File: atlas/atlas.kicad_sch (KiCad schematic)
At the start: 0 parts

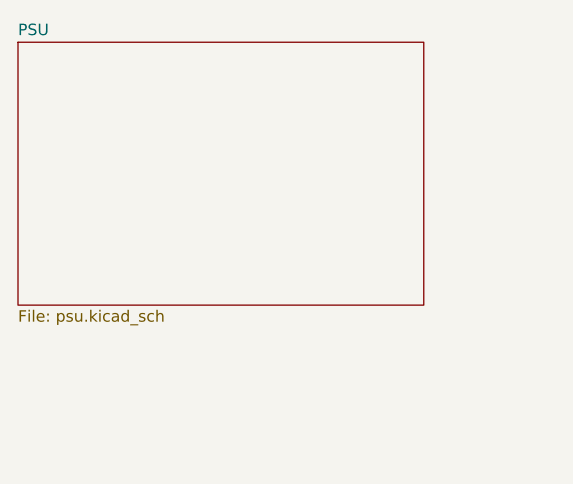
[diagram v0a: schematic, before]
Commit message: sensor supply
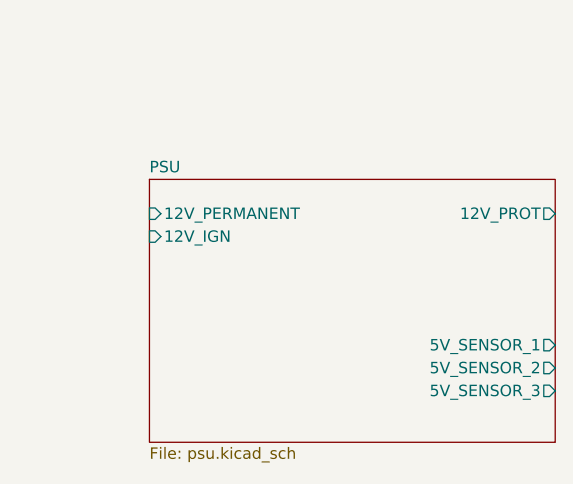
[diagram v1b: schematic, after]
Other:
- sheet PSU ports: added 12V_IGN, 12V_PERMANENT, 12V_PROT, 5V_SENSOR_1, 5V_SENSOR_2, 5V_SENSOR_3; removed none
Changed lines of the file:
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@@
     (rev "a")
   )
-  (sheet (at 20.32 17.78) (size 45.085 29.21) (fields_autoplaced)
+  (sheet (at 34.925 33.02) (size 45.085 29.21) (fields_autoplaced)
     (stroke (width 0.0006) (type solid) (color 0 0 0 0))
     (fill (color 0 0 0 0.0000))
-    (property "Sheet name" "PSU" (id 0) (at 20.32 17.1443 0)
+    (property "Sheet name" "PSU" (id 0) (at 34.925 32.3843 0)
       (effects (font (size 1.27 1.27)) (justify left bottom))
     )
-    (property "Sheet file" "psu.kicad_sch" (id 1) (at 20.32 47.4987 0)
+    (property "Sheet file" "psu.kicad_sch" (id 1) (at 34.925 62.7387 0)
       (effects (font (size 1.27 1.27)) (justify left top))
+    )
+    (pin "12V_PERMANENT" input (at 34.925 36.83 180)
+      (effects (font (size 1.27 1.27)) (justify left))
+    )
+    (pin "12V_IGN" input (at 34.925 39.37 180)
+      (effects (font (size 1.27 1.27)) (justify left))
+    )
+    (pin "12V_PROT" output (at 80.01 36.83 0)
+      (effects (font (size 1.27 1.27)) (justify right))
+    )
+    (pin "5V_SENSOR_1" output (at 80.01 51.435 0)
+      (effects (font (size 1.27 1.27)) (justify right))
+    )
+    (pin "5V_SENSOR_3" output (at 80.01 56.515 0)
+      (effects (font (size 1.27 1.27)) (justify right))
+    )
+    (pin "5V_SENSOR_2" output (at 80.01 53.975 0)
+      (effects (font (size 1.27 1.27)) (justify right))
     )
   )
@@
       (reference "#PWR0118") (unit 1) (value "GND") (footprint "")
     )
+    (path "/105389e3-dfa9-494e-826b-71f0b7c57c75/0967bfe0-49b2-41f4-aa5d-9a385ee45cf4"
+      (reference "#PWR?") (unit 1) (value "GND") (footprint "")
+    )
+    (path "/105389e3-dfa9-494e-826b-71f0b7c57c75/0b522575-1719-4a5f-9cab-c14ad8c11d8a"
+      (reference "#PWR?") (unit 1) (value "GND") (footprint "")
+    )
+    (path "/105389e3-dfa9-494e-826b-71f0b7c57c75/12d659ac-096d-4239-8e7f-b8bb10c7928c"
+      (reference "#PWR?") (unit 1) (value "GND") (footprint "")
+    )
+    (path "/105389e3-dfa9-494e-826b-71f0b7c57c75/1472509d-926b-44aa-92cc-99ec30a17c06"
+      (reference "#PWR?") (unit 1) (value "+5V") (footprint "")
+    )
+    (path "/105389e3-dfa9-494e-826b-71f0b7c57c75/2af3994e-4ff4-4fd7-9c3f-1fd5849c37b2"
+      (reference "#PWR?") (unit 1) (value "GND") (footprint "")
+    )
+    (path "/105389e3-dfa9-494e-826b-71f0b7c57c75/2c7c70f6-cc68-4362-b58f-d384cb3b9347"
+      (reference "#PWR?") (unit 1) (value "GND") (footprint "")
+    )
+    (path "/105389e3-dfa9-494e-826b-71f0b7c57c75/4e95f0b1-6137-4fa1-9ec8-25978a274a11"
+      (reference "#PWR?") (unit 1) (value "GND") (footprint "")
+    )
+    (path "/105389e3-dfa9-494e-826b-71f0b7c57c75/5f0ee79c-d992-4278-83c7-0dd3ff03258b"
+      (reference "#PWR?") (unit 1) (value "GND") (footprint "")
+    )
+    (path "/105389e3-dfa9-494e-826b-71f0b7c57c75/60ca8900-e57f-4a56-adcc-b0810fa493d7"
+      (reference "#PWR?") (unit 1) (value "GND") (footprint "")
+    )
+    (path "/105389e3-dfa9-494e-826b-71f0b7c57c75/8624984f-ec35-4738-9181-a62155e79137"
+      (reference "#PWR?") (unit 1) (value "+5V") (footprint "")
+    )
+    (path "/105389e3-dfa9-494e-826b-71f0b7c57c75/962a942a-c800-4bb9-b30c-312e7c0fc363"
+      (reference "#PWR?") (unit 1) (value "GND") (footprint "")
+    )
+    (path "/105389e3-dfa9-494e-826b-71f0b7c57c75/be890bbf-1bee-4e3d-8817-dbaa4bed2866"
+      (reference "#PWR?") (unit 1) (value "GND") (footprint "")
+    )
+    (path "/105389e3-dfa9-494e-826b-71f0b7c57c75/f2510f10-6daf-498f-863a-a83895bbf474"
+      (reference "#PWR?") (unit 1) (value "+5V") (footprint "")
+    )
     (path "/105389e3-dfa9-494e-826b-71f0b7c57c75/02fc3a4a-be60-43a8-bd44-462d111535eb"
       (reference "C?") (unit 1) (value "1u") (footprint "")
@@
       (reference "C?") (unit 1) (value "56u") (footprint "")
     )
+    (path "/105389e3-dfa9-494e-826b-71f0b7c57c75/3c027b09-5951-4b1a-bb22-246e74e92095"
+      (reference "C?") (unit 1) (value "1u") (footprint "")
+    )
     (path "/105389e3-dfa9-494e-826b-71f0b7c57c75/3fa14d60-e938-4069-8740-629d7edacfcd"
       (reference "C?") (unit 1) (value "10n") (footprint "")
@@
       (reference "C?") (unit 1) (value "270p") (footprint "")
     )
+    (path "/105389e3-dfa9-494e-826b-71f0b7c57c75/5cef4001-842d-4fec-89cb-073339ac197a"
+      (reference "C?") (unit 1) (value "C") (footprint "")
+    )
     (path "/105389e3-dfa9-494e-826b-71f0b7c57c75/7293eb0a-aafb-4ea9-ba5c-e3ef1261a7a6"
       (reference "C?") (unit 1) (value "1u") (footprint "")
@@
       (reference "C?") (unit 1) (value "33u") (footprint "")
     )
+    (path "/105389e3-dfa9-494e-826b-71f0b7c57c75/848680d5-6f8c-408c-bf57-0699581ce54b"
+      (reference "C?") (unit 1) (value "C") (footprint "")
+    )
     (path "/105389e3-dfa9-494e-826b-71f0b7c57c75/87a30954-7839-4868-b5d8-1ee1338cc331"
       (reference "C?") (unit 1) (value "100n") (footprint "")
@@
       (reference "C?") (unit 1) (value "4.7u") (footprint "")
     )
+    (path "/105389e3-dfa9-494e-826b-71f0b7c57c75/bafe5152-f260-4eb5-953c-9865271e4497"
+      (reference "C?") (unit 1) (value "C") (footprint "")
+    )
+    (path "/105389e3-dfa9-494e-826b-71f0b7c57c75/bfcb4021-49a9-43a2-8acc-f0e08c972e2d"
+      (reference "C?") (unit 1) (value "1u") (footprint "")
+    )
+    (path "/105389e3-dfa9-494e-826b-71f0b7c57c75/c3826fe4-fa0a-46e0-97ea-51363766c939"
+      (reference "C?") (unit 1) (value "1u") (footprint "")
+    )
     (path "/105389e3-dfa9-494e-826b-71f0b7c57c75/c515180a-c2d0-4ce1-9b80-ec2d8d3bb1fb"
       (reference "C?") (unit 1) (value "56u") (footprint "")
@@
       (reference "D?") (unit 1) (value "D_Schottky") (footprint "")
     )
+    (path "/105389e3-dfa9-494e-826b-71f0b7c57c75/5ab4a96f-3722-4728-9d80-3d7f6a1f649e"
+      (reference "D?") (unit 1) (value "D_Schottky") (footprint "")
+    )
     (path "/105389e3-dfa9-494e-826b-71f0b7c57c75/79ed81d4-2ba0-42b4-b1d9-789da637b797"
       (reference "D?") (unit 1) (value "5.1v") (footprint "")
     )
     (path "/105389e3-dfa9-494e-826b-71f0b7c57c75/1ed43776-d526-4a51-977e-cd7a4e2b67d4"
-      (reference "L?") (unit 1) (value "L") (footprint "")
+      (reference "L?") (unit 1) (value "10u") (footprint "")
     )
     (path "/105389e3-dfa9-494e-826b-71f0b7c57c75/b6743678-2084-4455-b6d4-1663b87e2da6"
@@
       (reference "R?") (unit 1) (value "10k") (footprint "")
     )
+    (path "/105389e3-dfa9-494e-826b-71f0b7c57c75/16fe8ffe-f8db-4475-97fa-418dfcbda05c"
+      (reference "U?") (unit 1) (value "TLS115D0EJ") (footprint "")
+    )
+    (path "/105389e3-dfa9-494e-826b-71f0b7c57c75/d440efdf-37c5-49ba-aa64-2abea4dfc6b9"
+      (reference "U?") (unit 1) (value "TLS115D0EJ") (footprint "")
+    )
     (path "/105389e3-dfa9-494e-826b-71f0b7c57c75/dfa577ab-9946-4a57-a6cf-e47b58bdffd1"
       (reference "U?") (unit 1) (value "LMR14020") (footprint "")
     )
-  )
+    (path "/105389e3-dfa9-494e-826b-71f0b7c57c75/ef1c8b94-6884-4b91-843e-9f78e79e2420"
+      (reference "U?") (unit 1) (value "TLS115D0EJ") (footprint "")
+    )
+  )
